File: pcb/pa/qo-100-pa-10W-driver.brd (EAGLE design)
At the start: 80 x 40 mm, 1 part

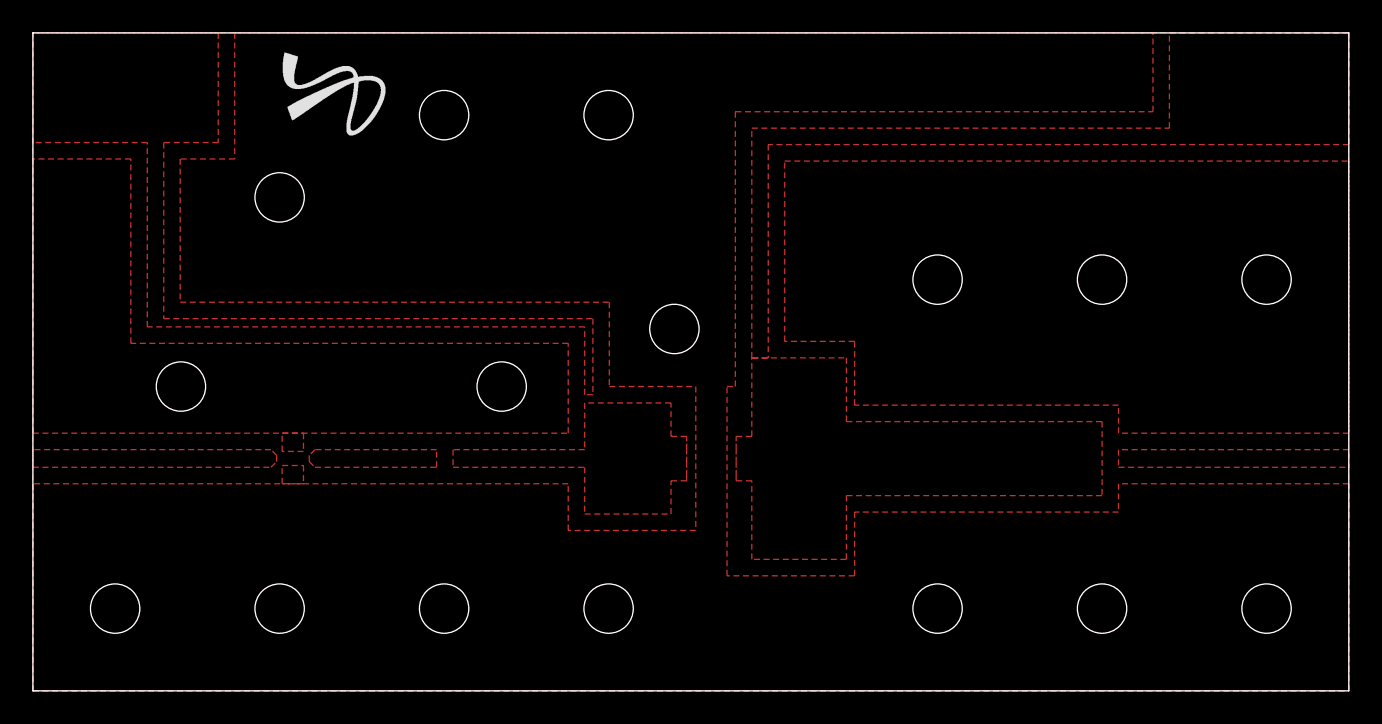
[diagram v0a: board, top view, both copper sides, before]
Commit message: Update PA PCBs
Signed-off-by: João Silva <jgc3silva@gmail.com>
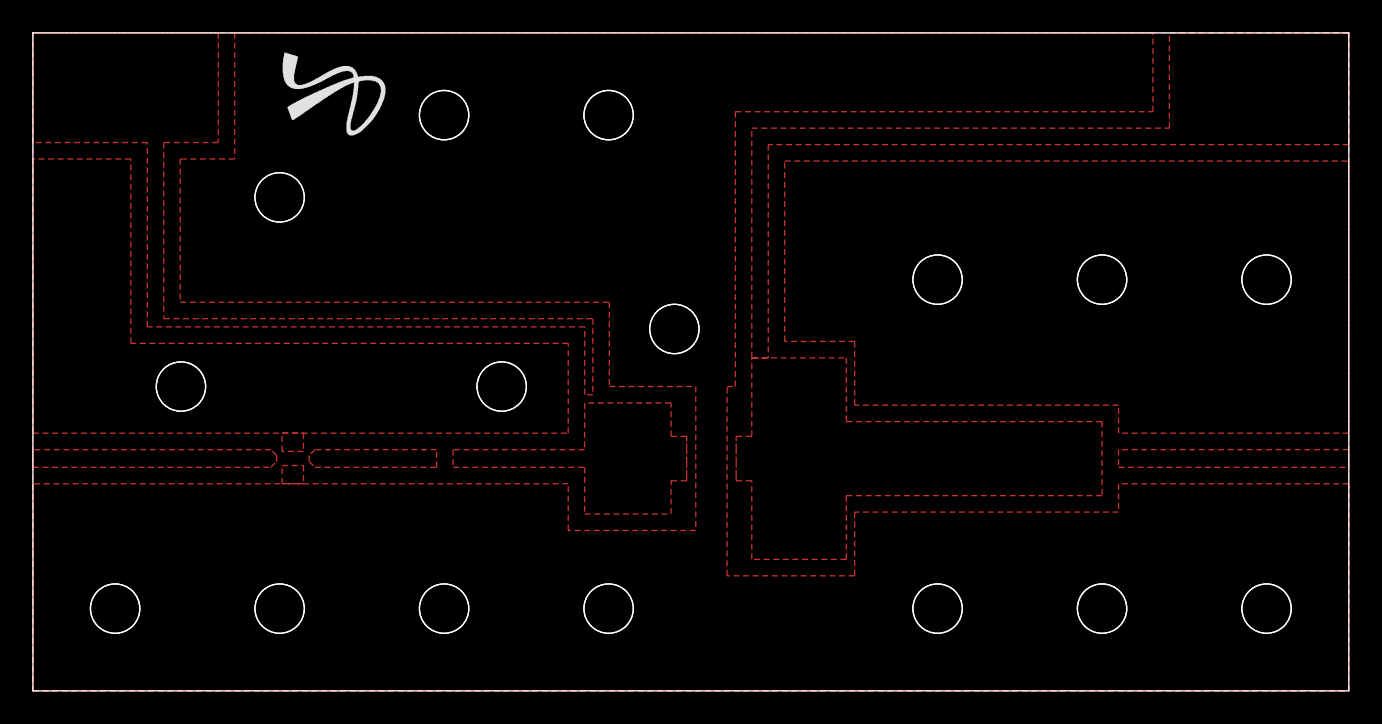
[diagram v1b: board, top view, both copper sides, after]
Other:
- outline, holes or cut-outs redrawn
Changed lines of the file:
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@@
 <setting verticaltext="up"/>
 </settings>
-<grid distance="1" unitdist="mm" unit="mm" style="lines" multiple="1" display="yes" altdistance="5" altunitdist="mil" altunit="mil"/>
+<grid distance="0.5" unitdist="mm" unit="mm" style="lines" multiple="1" display="yes" altdistance="5" altunitdist="mil" altunit="mil"/>
 <layers>
 <layer number="1" name="Top" color="4" fill="1" visible="yes" active="yes"/>
@@
 <hole x="55" y="5" drill="3"/>
 <hole x="39" y="22" drill="3"/>
+<circle x="9" y="18.5" radius="1.5" width="0" layer="20"/>
+<circle x="15" y="30" radius="1.5" width="0" layer="20"/>
+<circle x="25" y="35" radius="1.5" width="0" layer="20"/>
+<circle x="35" y="35" radius="1.5" width="0" layer="20"/>
+<circle x="39" y="22" radius="1.5" width="0" layer="20"/>
+<circle x="55" y="25" radius="1.5" width="0" layer="20"/>
+<circle x="65" y="25" radius="1.5" width="0" layer="20"/>
+<circle x="75" y="25" radius="1.5" width="0" layer="20"/>
+<circle x="75" y="5" radius="1.5" width="0" layer="20"/>
+<circle x="65" y="5" radius="1.5" width="0" layer="20"/>
+<circle x="55" y="5" radius="1.5" width="0" layer="20"/>
+<circle x="35" y="5" radius="1.5" width="0" layer="20"/>
+<circle x="25" y="5" radius="1.5" width="0" layer="20"/>
+<circle x="15" y="5" radius="1.5" width="0" layer="20"/>
+<circle x="28.5" y="18.5" radius="1.5" width="0" layer="20"/>
+<circle x="5" y="5" radius="1.5" width="0" layer="20"/>
 </plain>
 <attributes>
